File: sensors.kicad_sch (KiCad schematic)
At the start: 19 parts, among them J3 CONMHF1-SMD-G-T, U19 LSM6DSOXTR, U2 AK09940A, U3 ICM-42688-P, U4 ICM-45686, U5 DPS368XTSA1, U9 MAX-M10S

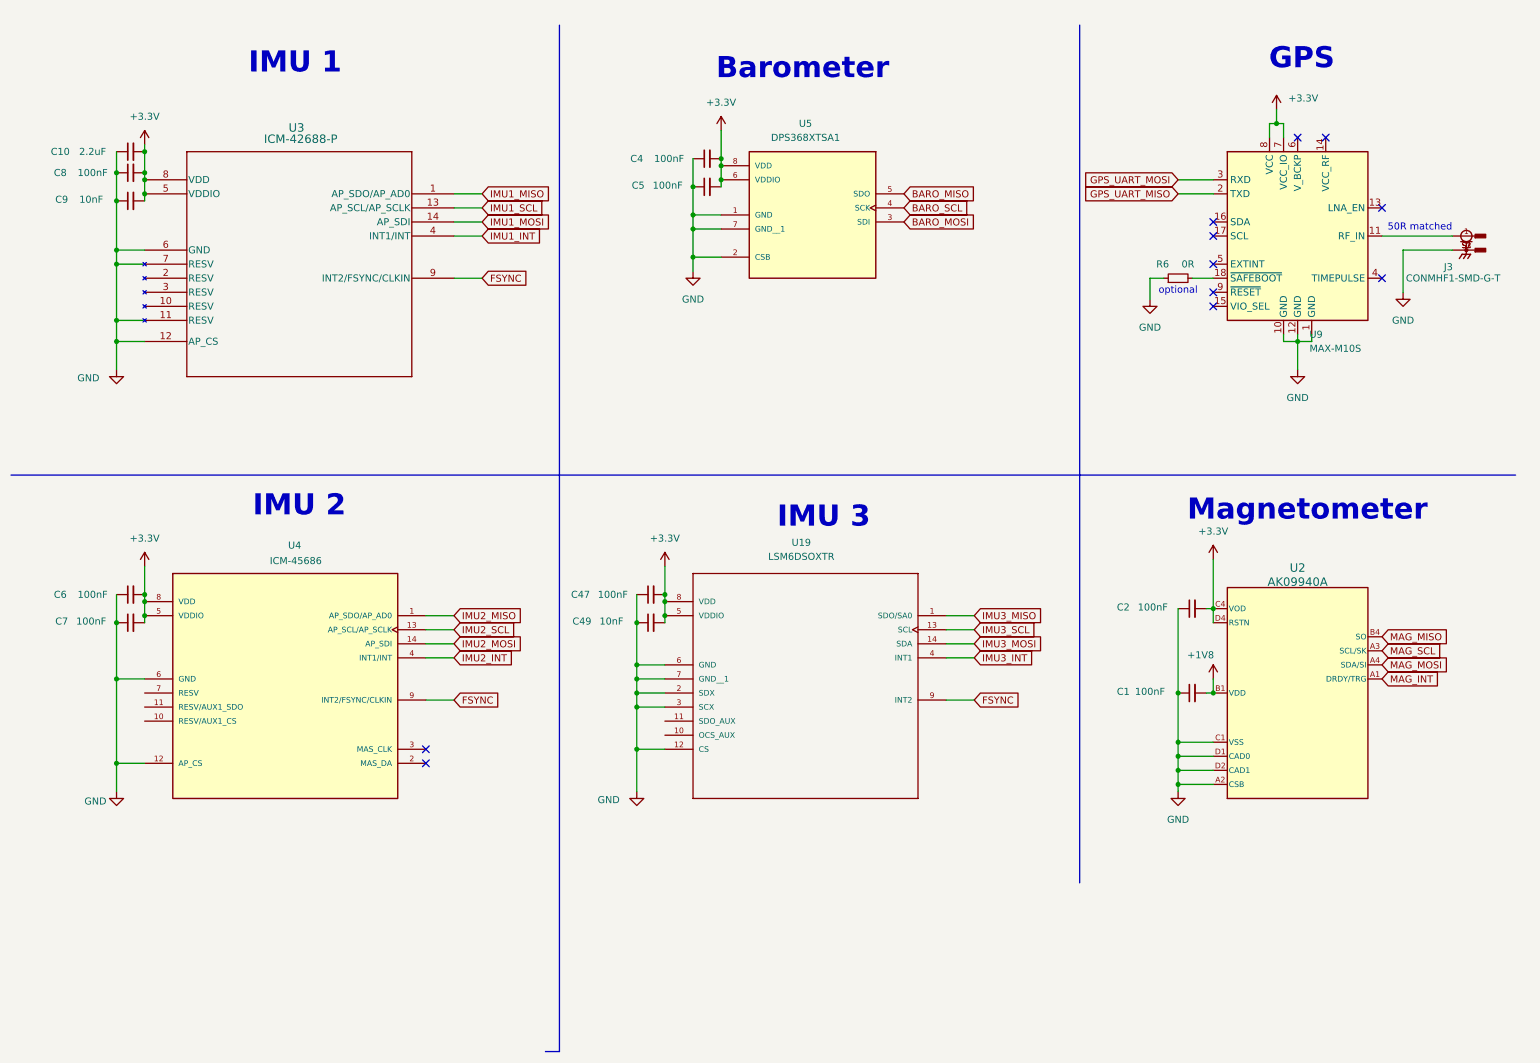
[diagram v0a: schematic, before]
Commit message: V2 with feedback
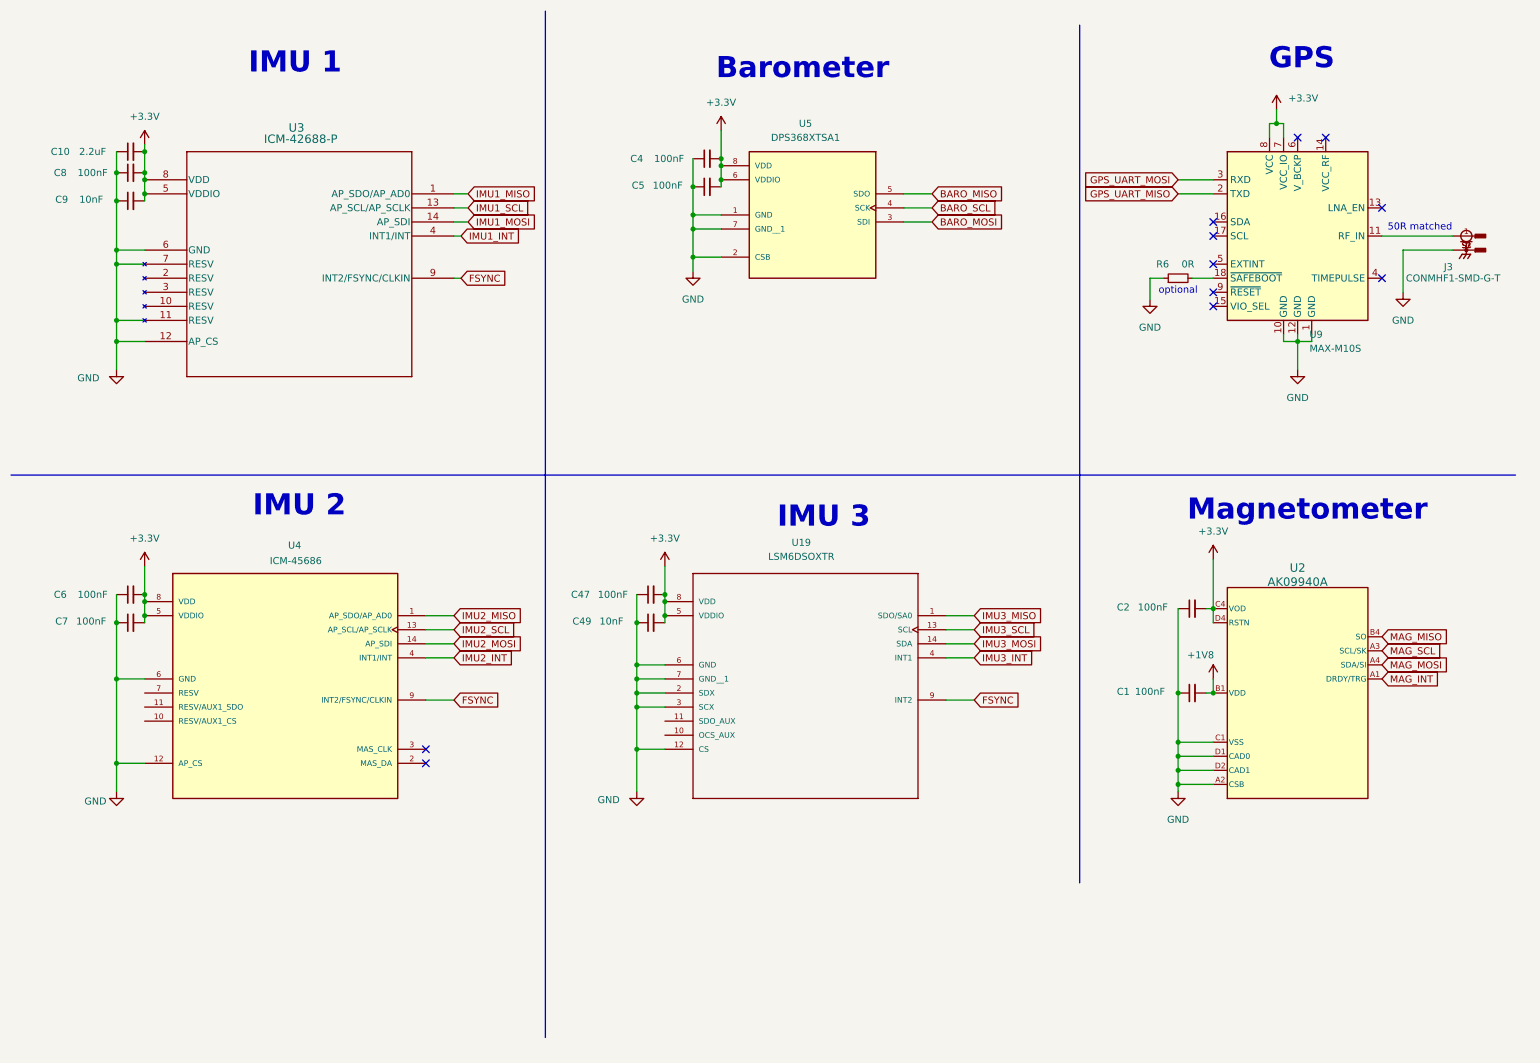
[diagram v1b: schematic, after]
